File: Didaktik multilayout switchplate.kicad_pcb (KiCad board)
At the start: 2 copper layers, 209.6 x 85.9 mm, 0 parts

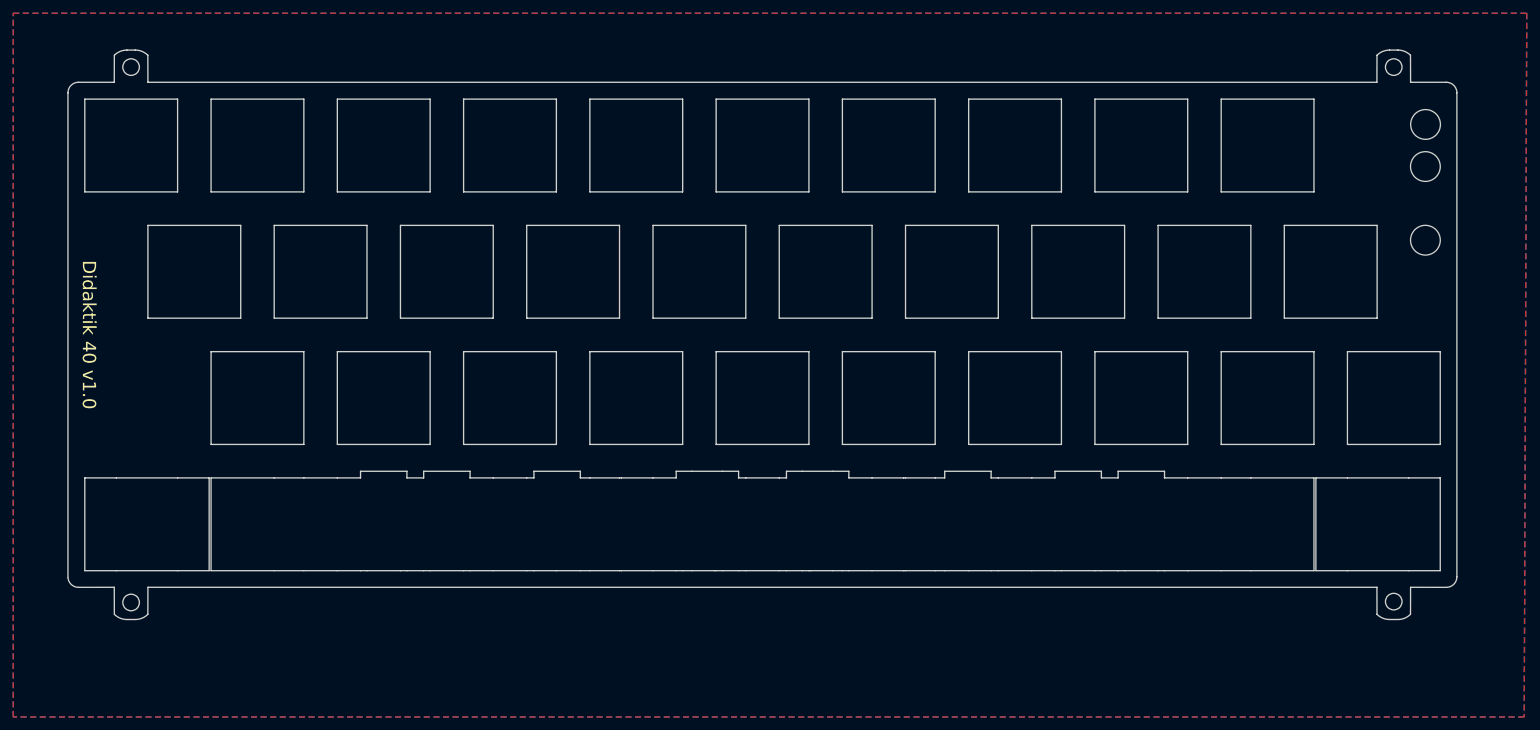
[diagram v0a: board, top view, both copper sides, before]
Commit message: production files
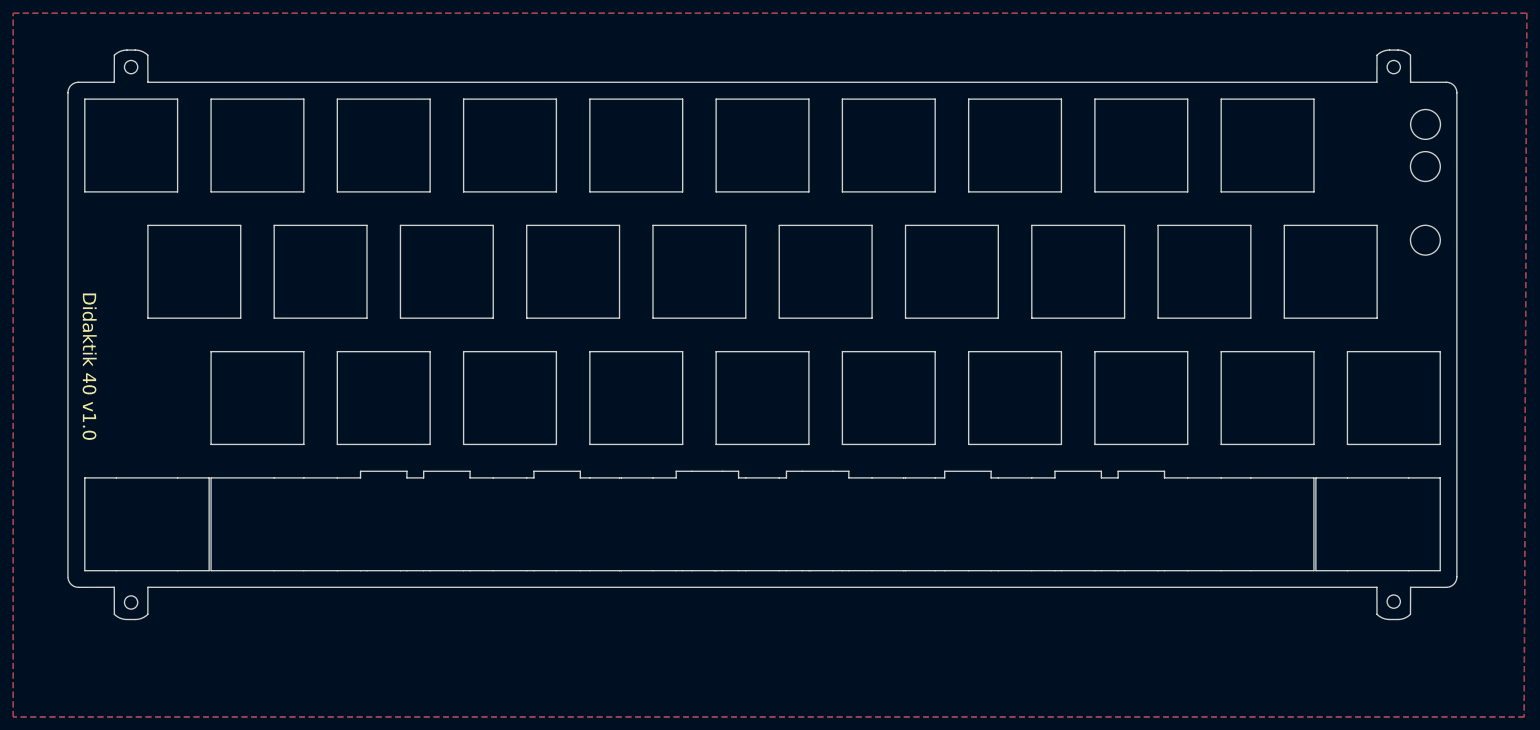
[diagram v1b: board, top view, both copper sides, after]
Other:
- outline, holes or cut-outs redrawn
- board text added: "screwholes m2"
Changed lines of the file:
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@@
       (outputformat 1)
       (mirror false)
-      (drillshape 1)
+      (drillshape 0)
       (scaleselection 1)
-      (outputdirectory "")
+      (outputdirectory "Production/Plate")
     )
   )
@@
   (gr_line (start 62.865 67.34) (end 76.865 67.34) (layer "Edge.Cuts") (width 0.2))
   (gr_line (start 53.34 48.29) (end 67.34 48.29) (layer "Edge.Cuts") (width 0.2))
-  (gr_circle (center 236.572361 38.112584) (end 238.817425 38.112584) (layer "Edge.Cuts") (width 0.1) (fill none))
+  (gr_circle (center 236.572361 38.112584) (end 238.822361 38.112584) (layer "Edge.Cuts") (width 0.2) (fill none))
   (gr_line (start 164.028 105.44) (end 167.64 105.44) (layer "Edge.Cuts") (width 0.2))
   (gr_line (start 40.639355 26.891284) (end 41.909355 26.891284) (layer "Edge.Cuts") (width 0.2))
@@
   (gr_line (start 102.052 90.44) (end 102.052 91.44) (layer "Edge.Cuts") (width 0.2))
   (gr_line (start 57.815 53.34) (end 43.815 53.34) (layer "Edge.Cuts") (width 0.2))
-  (gr_circle (center 236.549797 44.462584) (end 238.794861 44.462584) (layer "Edge.Cuts") (width 0.1) (fill none))
+  (gr_circle (center 236.549797 44.462584) (end 238.799797 44.462584) (layer "Edge.Cuts") (width 0.2) (fill none))
   (gr_line (start 134.015 53.34) (end 120.015 53.34) (layer "Edge.Cuts") (width 0.2))
   (gr_line (start 85.415 90.44) (end 85.415 91.44) (layer "Edge.Cuts") (width 0.2))
@@
   (gr_line (start 210.215 105.44) (end 219.74 105.44) (layer "Edge.Cuts") (width 0.2))
   (gr_line (start 143.54 105.44) (end 143.8275 105.44) (layer "Edge.Cuts") (width 0.2))
-  (gr_circle (center 231.775 110.103387) (end 233.025 110.103387) (layer "Edge.Cuts") (width 0.2) (fill none))
+  (gr_circle (center 231.775 110.103387) (end 232.775 110.103387) (layer "Edge.Cuts") (width 0.2) (fill none))
   (gr_line (start 158.115 105.44) (end 162.59 105.44) (layer "Edge.Cuts") (width 0.2))
   (gr_line (start 132.928 90.44) (end 130.515 90.44) (layer "Edge.Cuts") (width 0.2))
@@
   (gr_line (start 224.79 91.44) (end 220.0275 91.44) (layer "Edge.Cuts") (width 0.2))
   (gr_line (start 132.928 91.44) (end 132.928 90.44) (layer "Edge.Cuts") (width 0.2))
-  (gr_circle (center 236.5525 55.5775) (end 238.14 57.165) (layer "Edge.Cuts") (width 0.1) (fill none))
+  (gr_circle (center 236.5525 55.5775) (end 238.8025 55.5775) (layer "Edge.Cuts") (width 0.2) (fill none))
   (gr_line (start 132.928 105.44) (end 134.015 105.44) (layer "Edge.Cuts") (width 0.2))
   (gr_line (start 38.749134 112.019614) (end 38.735 107.944387) (layer "Edge.Cuts") (width 0.2))
@@
   (gr_line (start 219.74 72.39) (end 205.74 72.39) (layer "Edge.Cuts") (width 0.2))
   (gr_line (start 53.34 105.44) (end 62.865 105.44) (layer "Edge.Cuts") (width 0.2))
-  (gr_circle (center 41.275 29.458387) (end 40.025 29.458387) (layer "Edge.Cuts") (width 0.2) (fill none))
+  (gr_circle (center 41.275 29.458387) (end 42.275 29.458387) (layer "Edge.Cuts") (width 0.2) (fill none))
   (gr_line (start 200.69 86.39) (end 200.69 72.39) (layer "Edge.Cuts") (width 0.2))
   (gr_line (start 181.64 72.39) (end 167.64 72.39) (layer "Edge.Cuts") (width 0.2))
@@
   (gr_line (start 48.29 105.44) (end 53.0525 105.44) (layer "Edge.Cuts") (width 0.2))
   (gr_line (start 219.74 91.44) (end 210.215 91.44) (layer "Edge.Cuts") (width 0.2))
-  (gr_circle (center 231.775 29.458387) (end 230.525 29.458387) (layer "Edge.Cuts") (width 0.2) (fill none))
+  (gr_circle (center 231.775 29.458387) (end 232.775 29.458387) (layer "Edge.Cuts") (width 0.2) (fill none))
   (gr_line (start 205.74 72.39) (end 205.74 86.39) (layer "Edge.Cuts") (width 0.2))
   (gr_line (start 231.139355 26.891284) (end 232.409355 26.891284) (layer "Edge.Cuts") (width 0.2))
@@
   (gr_line (start 43.814355 31.75) (end 229.235 31.75) (layer "Edge.Cuts") (width 0.2))
   (gr_line (start 75.89 105.44) (end 76.865 105.44) (layer "Edge.Cuts") (width 0.2))
-  (gr_circle (center 41.275 110.236) (end 42.525 110.236) (layer "Edge.Cuts") (width 0.2) (fill none))
+  (gr_circle (center 41.275 110.236) (end 42.275 110.236) (layer "Edge.Cuts") (width 0.2) (fill none))
   (gr_line (start 123.515 90.44) (end 123.515 91.44) (layer "Edge.Cuts") (width 0.2))
   (gr_line (start 148.59 86.39) (end 162.59 86.39) (layer "Edge.Cuts") (width 0.2))
@@
   (gr_line (start 200.69 91.44) (end 197.19 91.44) (layer "Edge.Cuts") (width 0.2))
   (gr_arc (start 38.747844 27.674773) (mid 39.615675 27.094903) (end 40.639355 26.891284) (layer "Edge.Cuts") (width 0.2))
-  (gr_text "Didaktik 40 v1.0" (at 34.925 69.85 -90) (layer "F.SilkS")
+  (gr_text "Didaktik 40 v1.0" (at 34.925 74.6125 -90) (layer "F.SilkS")
     (effects (font (size 2 2) (thickness 0.15)))
   )
+  (gr_text "screwholes m2" (at 136.017 24.765) (layer "Cmts.User")
+    (effects (font (size 1.5 1.5) (thickness 0.3)))
+  )
   (dimension (type aligned) (layer "Cmts.User")
